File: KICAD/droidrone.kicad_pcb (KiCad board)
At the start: 2 copper layers, 100 x 50 mm, 72 parts, among them IC1 ATMEGA328PB, P1 USB_A, U1 LM7805CT, U4 LP2950L-3.3V, Y1 Crystal

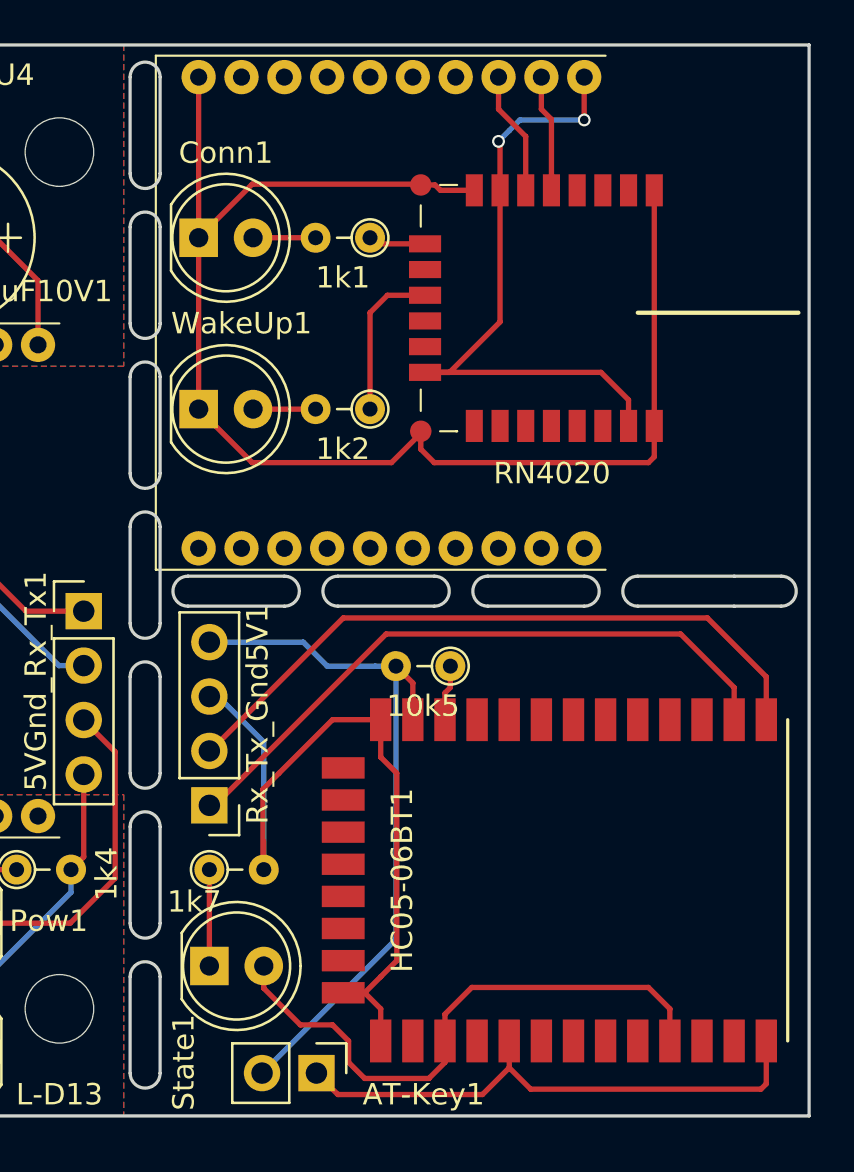
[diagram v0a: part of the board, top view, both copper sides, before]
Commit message: same fix.
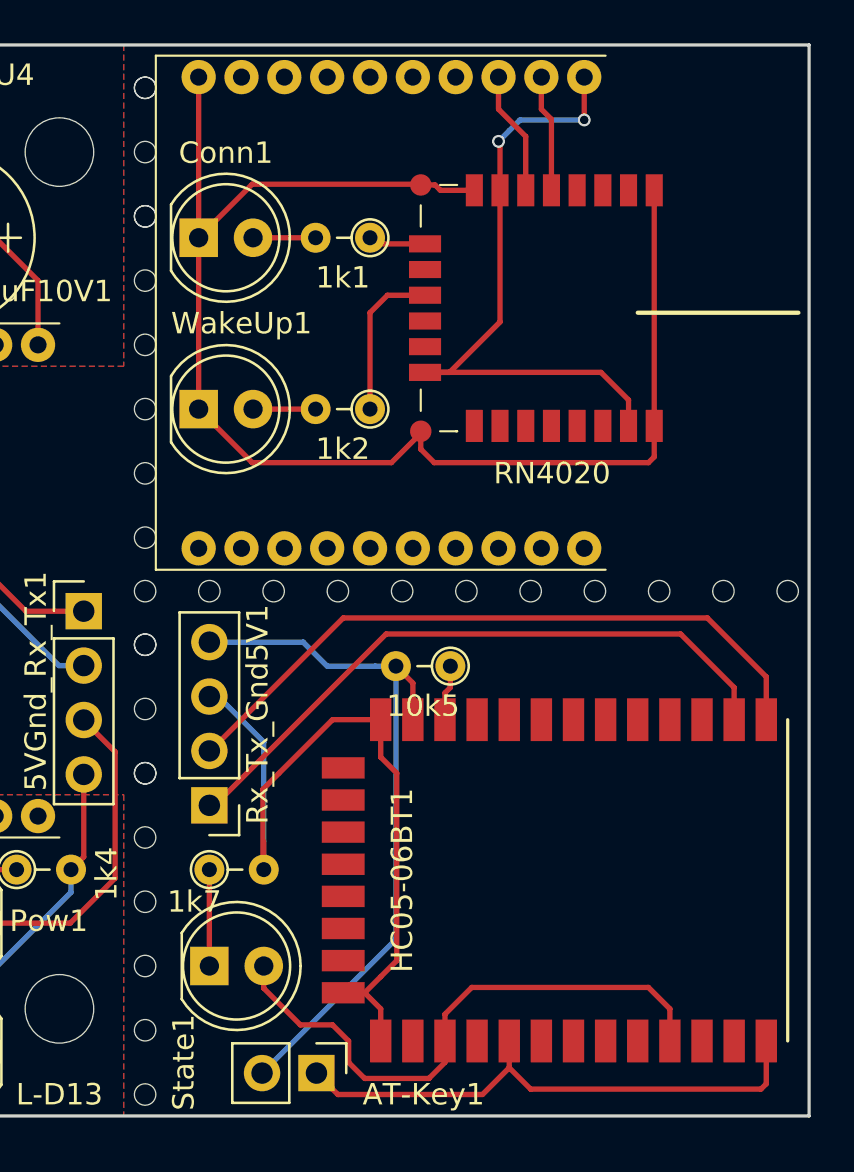
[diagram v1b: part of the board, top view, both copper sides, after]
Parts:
- added ?: Hole_1.0mm, lib:Hole_1.0mm, F.Cu at (224.0, 50.5)
- added ?: Hole_1.0mm, lib:Hole_1.0mm, F.Cu at (197.0, 50.5)
- added ? (x2): Hole_1.0mm, lib:Hole_1.0mm, F.Cu at (194.0, 53.0)
- added ?: Hole_1.0mm, lib:Hole_1.0mm, F.Cu at (194.0, 56.0)
- added ?: Hole_1.0mm, lib:Hole_1.0mm, F.Cu at (194.0, 74.0)
- added ?: Hole_1.0mm, lib:Hole_1.0mm, F.Cu at (194.0, 71.0)
- added ?: Hole_1.0mm, lib:Hole_1.0mm, F.Cu at (194.0, 65.0)
- added ?: Hole_1.0mm, lib:Hole_1.0mm, F.Cu at (194.0, 68.0)
- added ?: Hole_1.0mm, lib:Hole_1.0mm, F.Cu at (194.0, 62.0)
- added ? (x2): Hole_1.0mm, lib:Hole_1.0mm, F.Cu at (194.0, 59.0)
- added ?: Hole_1.0mm, lib:Hole_1.0mm, F.Cu at (221.0, 50.5)
- added ? (x2): Hole_1.0mm, lib:Hole_1.0mm, F.Cu at (194.0, 33.0)
- added ?: Hole_1.0mm, lib:Hole_1.0mm, F.Cu at (194.0, 36.0)
- added ?: Hole_1.0mm, lib:Hole_1.0mm, F.Cu at (194.0, 42.0)
- added ?: Hole_1.0mm, lib:Hole_1.0mm, F.Cu at (194.0, 39.0)
- added ?: Hole_1.0mm, lib:Hole_1.0mm, F.Cu at (194.0, 45.0)
- added ?: Hole_1.0mm, lib:Hole_1.0mm, F.Cu at (194.0, 48.0)
- added ?: Hole_1.0mm, lib:Hole_1.0mm, F.Cu at (194.0, 50.5)
- added ?: Hole_1.0mm, lib:Hole_1.0mm, F.Cu at (194.0, 30.0)
- added ?: Hole_1.0mm, lib:Hole_1.0mm, F.Cu at (218.0, 50.5)
- added ? (x2): Hole_1.0mm, lib:Hole_1.0mm, F.Cu at (194.0, 27.0)
- added ?: Hole_1.0mm, lib:Hole_1.0mm, F.Cu at (206.0, 50.5)
- added ?: Hole_1.0mm, lib:Hole_1.0mm, F.Cu at (209.0, 50.5)
- added ?: Hole_1.0mm, lib:Hole_1.0mm, F.Cu at (215.0, 50.5)
- added ?: Hole_1.0mm, lib:Hole_1.0mm, F.Cu at (212.0, 50.5)
- added ?: Hole_1.0mm, lib:Hole_1.0mm, F.Cu at (200.0, 50.5)
- added ?: Hole_1.0mm, lib:Hole_1.0mm, F.Cu at (203.0, 50.5)
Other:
- outline, holes or cut-outs redrawn
